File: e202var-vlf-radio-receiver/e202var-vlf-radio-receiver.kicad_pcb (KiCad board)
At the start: 2 copper layers, 55.9 x 81.3 mm, 49 parts, among them J1 9V, J2 ON/OFF, J3 HEADPHONES, J4 12V/18V, J5 FILTER, Q1 BC547, Q2 BC547, U1 MC7809, U2 TLE2426, U3 NJM386, U4 TL081CP

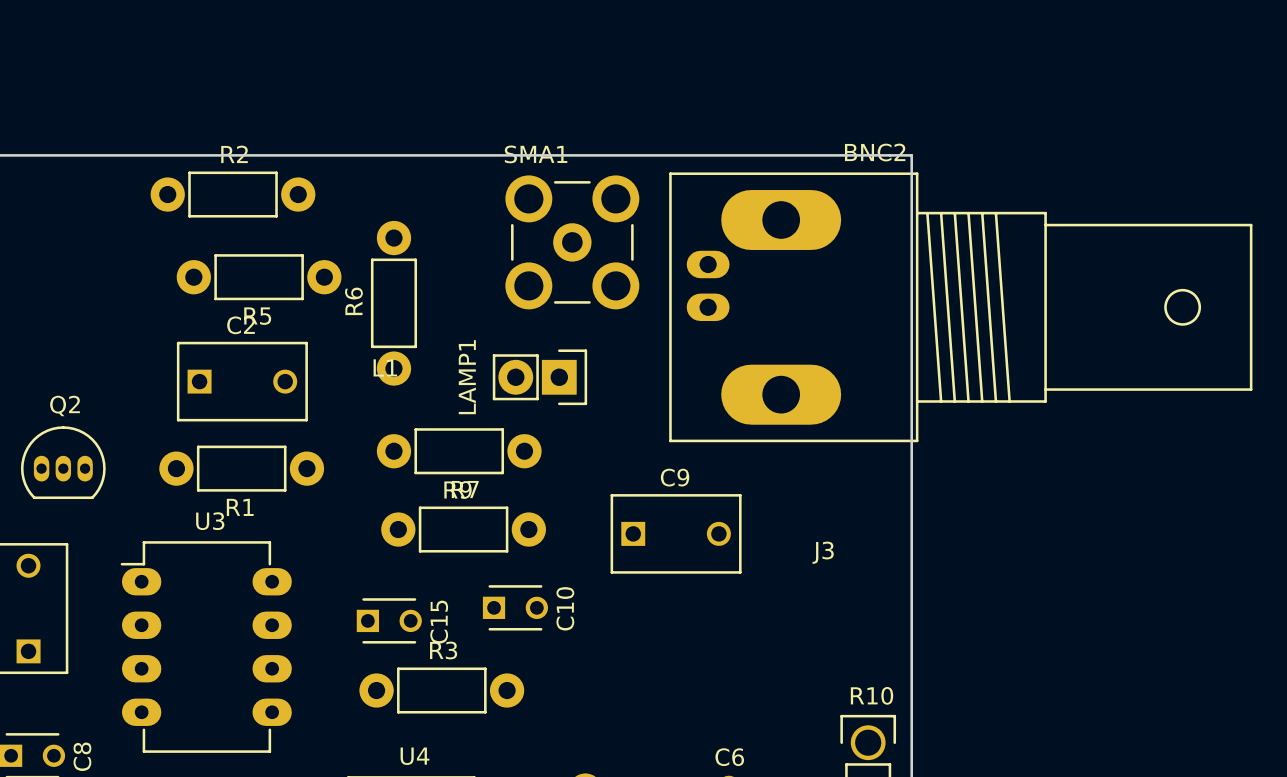
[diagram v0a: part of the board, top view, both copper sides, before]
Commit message: Added parts. Ready for layout.
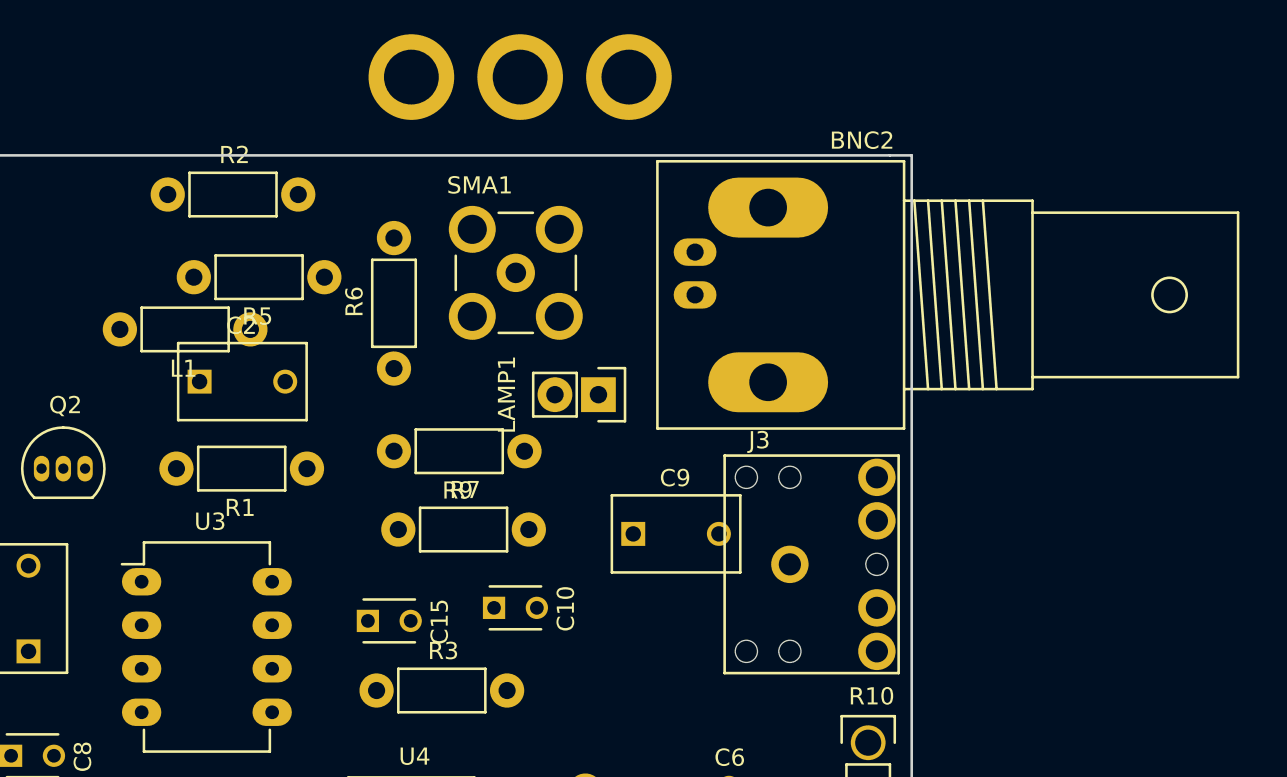
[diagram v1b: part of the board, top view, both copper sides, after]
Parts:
- added REF**: HOLE-PLATED-3.2MM, Wickerlib:HOLE-PLATED-3.2MM, F.Cu at (85.1, 33.5)
- added REF**: HOLE-PLATED-3.2MM, Wickerlib:HOLE-PLATED-3.2MM, F.Cu at (91.4, 33.5)
- added REF**: HOLE-PLATED-3.2MM, Wickerlib:HOLE-PLATED-3.2MM, F.Cu at (97.8, 33.5)
- L1: footprint Wickerlib:IND-78F-AXIAL -> Wickerlib:RES-CARBONFILM-7MM
- moved J3 4.32 mm to (107.2, 64.5)
- moved SMA1 3.75 mm to (91.2, 45.0)
- moved L1 2.65 mm to (75.7, 48.3), turned to 180 degrees
- moved LAMP1 2.50 mm to (96.0, 52.1)
- moved BNC2 1.05 mm to (106.7, 46.2)
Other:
- board text added: "12/9/2016"
- board text added: "E202VAR VLF Natural Radio Receiver"
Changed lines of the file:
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@@
 (kicad_pcb (version 4) (host pcbnew 4.0.4+e1-6308~48~ubuntu16.04.1-stable)
   (general
-    (links 87)
-    (no_connects 87)
-    (area 0 0 0 0)
+    (links 94)
+    (no_connects 94)
+    (area 58.343799 38.023799 114.376201 119.456201)
     (thickness 1.6)
-    (drawings 22)
+    (drawings 28)
     (tracks 0)
     (zones 0)
-    (modules 49)
+    (modules 52)
     (nets 33)
   )
@@
   )
   (module Wickerlib:CONN-BNC-TECONN-1-1634612-0 (layer F.Cu)
-    (at 107.4166 46.96968 270)
+    (at 106.6546 46.24578 270)
     (descr "BNC Socket TYCO AMP")
     (tags "BNC Socket TYCO AMP")
@@
       (net 29 "Net-(J1-Pad1)"))
   )
-  (module Wickerlib:SJ1-3523N (layer F.Cu)
-    (at 109.22 60.706)
-    (fp_text reference J3 (at 0 0.5) (layer F.SilkS)
-      (effects (font (size 1 1) (thickness 0.15)))
-    )
-    (fp_text value HEADPHONES (at 0 -0.5) (layer F.Fab)
-      (effects (font (size 1 1) (thickness 0.15)))
-    )
-  )
   (module Wickerlib:CONN-BARREL-JACK-2.5x5.5MM-TH (layer F.Cu)
     (at 90.651 109.5224 90)
@@
       (net 5 +2V))
   )
-  (module Wickerlib:IND-78F-AXIAL (layer F.Cu)
-    (at 76.454 50.8)
-    (fp_text reference L1 (at 7.112 -0.254) (layer F.SilkS)
-      (effects (font (size 1 1) (thickness 0.15)))
-    )
-    (fp_text value 3.3UH (at 0 -0.5) (layer F.Fab)
-      (effects (font (size 1 1) (thickness 0.15)))
-    )
-  )
   (module Wickerlib:CONN-HEADER-STRAIGHT-P2.54MM-1x02 (layer F.Cu)
-    (at 93.726 51.054 270)
+    (at 96.012 52.07 270)
     (descr "Through hole pin header")
     (tags "pin header")
@@
   )
   (module Wickerlib:CONN-SMA-STRAIGHT-TH (layer F.Cu)
-    (at 94.488 43.18)
+    (at 91.186 44.958)
     (descr "SMA pcb mounting jack")
     (tags "SMA Jack  Striaght")
@@
     (pad 8 thru_hole oval (at 7.62 0) (size 2.3 1.6) (drill 0.8) (layers *.Cu *.Mask F.SilkS))
   )
+  (module Wickerlib:RES-CARBONFILM-7MM (layer F.Cu)
+    (at 75.692 48.26 180)
+    (descr "Resistor, Axial,  RM 7.62mm, 1/3W,")
+    (tags "Resistor Axial RM 7.62mm 1/3W R3")
+    (fp_text reference L1 (at 3.8 0 180) (layer F.Fab)
+      (effects (font (size 1 1) (thickness 0.15)))
+    )
+    (fp_text value 3.3UH (at 3.81 3.81 180) (layer F.Fab) hide
+      (effects (font (size 1 1) (thickness 0.15)))
+    )
+    (fp_text user %R (at 3.9 -2.3 180) (layer F.SilkS)
+      (effects (font (size 1 1) (thickness 0.15)))
+    )
+    (fp_line (start 8.9 -1.5) (end -1.3 -1.5) (layer F.Fab) (width 0.0508))
+    (fp_line (start 8.9 1.5) (end 8.9 -1.5) (layer F.Fab) (width 0.0508))
+    (fp_line (start 8.8 1.5) (end 8.9 1.5) (layer F.Fab) (width 0.0508))
+    (fp_line (start -1.3 1.5) (end 8.8 1.5) (layer F.Fab) (width 0.0508))
+    (fp_line (start -1.3 -1.5) (end -1.3 1.5) (layer F.Fab) (width 0.0508))
+    (fp_line (start -1.25 -1.5) (end 8.85 -1.5) (layer F.CrtYd) (width 0.05))
+    (fp_line (start -1.25 1.5) (end -1.25 -1.5) (layer F.CrtYd) (width 0.05))
+    (fp_line (start 8.85 -1.5) (end 8.85 1.5) (layer F.CrtYd) (width 0.05))
+    (fp_line (start -1.25 1.5) (end 8.85 1.5) (layer F.CrtYd) (width 0.05))
+    (fp_line (start 1.27 -1.27) (end 6.35 -1.27) (layer F.SilkS) (width 0.15))
+    (fp_line (start 6.35 -1.27) (end 6.35 1.27) (layer F.SilkS) (width 0.15))
+    (fp_line (start 6.35 1.27) (end 1.27 1.27) (layer F.SilkS) (width 0.15))
+    (fp_line (start 1.27 1.27) (end 1.27 -1.27) (layer F.SilkS) (width 0.15))
+    (pad 1 thru_hole circle (at 0 0 180) (size 1.99898 1.99898) (drill 1.00076) (layers *.Cu *.SilkS *.Mask)
+      (net 3 "Net-(BNC2-Pad1)"))
+    (pad 2 thru_hole circle (at 7.62 0 180) (size 1.99898 1.99898) (drill 1.00076) (layers *.Cu *.SilkS *.Mask)
+      (net 7 "Net-(C2-Pad2)"))
+  )
+  (module Wickerlib:HOLE-PLATED-3.2MM (layer F.Cu)
+    (at 85.09 33.528)
+    (fp_text reference REF** (at 0 0) (layer F.Fab)
+      (effects (font (size 1 1) (thickness 0.15)))
+    )
+    (fp_text value HOLE-PLATED-3.2MM (at 0 -0.5) (layer F.Fab) hide
+      (effects (font (size 1 1) (thickness 0.15)))
+    )
+    (fp_circle (center 0 0) (end 2.54 1.27) (layer F.Fab) (width 0.04064))
+    (pad 1 thru_hole circle (at 0 0) (size 5 5) (drill 3.2) (layers *.Cu *.Mask))
+  )
+  (module Wickerlib:HOLE-PLATED-3.2MM (layer F.Cu)
+    (at 91.44 33.528)
+    (fp_text reference REF** (at 0 0) (layer F.Fab)
+      (effects (font (size 1 1) (thickness 0.15)))
+    )
+    (fp_text value HOLE-PLATED-3.2MM (at 0 -0.5) (layer F.Fab) hide
+      (effects (font (size 1 1) (thickness 0.15)))
+    )
+    (fp_circle (center 0 0) (end 2.54 1.27) (layer F.Fab) (width 0.04064))
+    (pad 1 thru_hole circle (at 0 0) (size 5 5) (drill 3.2) (layers *.Cu *.Mask))
+  )
+  (module Wickerlib:HOLE-PLATED-3.2MM (layer F.Cu)
+    (at 97.79 33.528)
+    (fp_text reference REF** (at 0 0) (layer F.Fab)
+      (effects (font (size 1 1) (thickness 0.15)))
+    )
+    (fp_text value HOLE-PLATED-3.2MM (at 0 -0.5) (layer F.Fab) hide
+      (effects (font (size 1 1) (thickness 0.15)))
+    )
+    (fp_circle (center 0 0) (end 2.54 1.27) (layer F.Fab) (width 0.04064))
+    (pad 1 thru_hole circle (at 0 0) (size 5 5) (drill 3.2) (layers *.Cu *.Mask))
+  )
+  (module Wickerlib:SJ1-3523N (layer F.Cu)
+    (at 107.188 64.516)
+    (fp_text reference J3 (at 1.27 -2.413) (layer F.Fab)
+      (effects (font (size 1 1) (thickness 0.15)))
+    )
+    (fp_text value HEADPHONES (at 0 -0.5) (layer F.Fab) hide
+      (effects (font (size 1 1) (thickness 0.15)))
+    )
+    (fp_text user %R (at -1.778 -9.779) (layer F.SilkS)
+      (effects (font (size 1 1) (thickness 0.15)))
+    )
+    (fp_line (start -3.81 3.81) (end 6.35 3.81) (layer F.CrtYd) (width 0.04064))
+    (fp_line (start -3.81 -8.89) (end -3.81 3.81) (layer F.CrtYd) (width 0.04064))
+    (fp_line (start 6.35 -8.89) (end -3.81 -8.89) (layer F.CrtYd) (width 0.04064))
+    (fp_line (start 6.35 3.81) (end 6.35 -8.89) (layer F.CrtYd) (width 0.04064))
+    (fp_line (start -3.81 3.81) (end 6.35 3.81) (layer F.Fab) (width 0.04064))
+    (fp_line (start -3.81 -8.89) (end -3.81 3.81) (layer F.Fab) (width 0.04064))
+    (fp_line (start 6.35 -8.89) (end -3.81 -8.89) (layer F.Fab) (width 0.04064))
+    (fp_line (start 6.35 -8.89) (end 6.35 3.81) (layer F.Fab) (width 0.04064))
+    (fp_line (start -3.81 3.81) (end 6.35 3.81) (layer F.SilkS) (width 0.1524))
+    (fp_line (start -3.81 -8.89) (end -3.81 3.81) (layer F.SilkS) (width 0.1524))
+    (fp_line (start 6.35 -8.89) (end -3.81 -8.89) (layer F.SilkS) (width 0.1524))
+    (fp_line (start 6.35 3.81) (end 6.35 -8.89) (layer F.SilkS) (width 0.1524))
+    (pad 4 thru_hole circle (at 5.08 -7.62) (size 2.1844 2.1844) (drill 1.2954) (layers *.Cu *.Mask)
+      (net 1 GND))
+    (pad 3 thru_hole circle (at 5.08 -5.08) (size 2.1844 2.1844) (drill 1.2954) (layers *.Cu *.Mask)
+      (net 1 GND))
+    (pad "" np_thru_hole circle (at 5.08 -2.54) (size 1.2954 1.2954) (drill 1.2954) (layers *.Cu))
+    (pad 2 thru_hole circle (at 5.08 0) (size 2.1844 2.1844) (drill 1.2954) (layers *.Cu *.Mask)
+      (net 17 "Net-(C9-Pad1)"))
+    (pad 1 thru_hole circle (at 5.08 2.54) (size 2.1844 2.1844) (drill 1.2954) (layers *.Cu *.Mask)
+      (net 17 "Net-(C9-Pad1)"))
+    (pad 5 thru_hole circle (at 0 -2.54) (size 2.1844 2.1844) (drill 1.2954) (layers *.Cu *.Mask)
+      (net 1 GND))
+    (pad "" np_thru_hole circle (at 0 -7.62) (size 1.2954 1.2954) (drill 1.2954) (layers *.Cu))
+    (pad "" np_thru_hole circle (at -2.54 -7.62) (size 1.2954 1.2954) (drill 1.2954) (layers *.Cu))
+    (pad "" np_thru_hole circle (at 0 2.54) (size 1.2954 1.2954) (drill 1.2954) (layers *.Cu))
+    (pad "" np_thru_hole circle (at -2.54 2.54) (size 1.2954 1.2954) (drill 1.2954) (layers *.Cu))
+  )
+  (gr_text 12/9/2016 (at 109.22 30.734) (layer F.Fab)
+    (effects (font (size 1.016 1.016) (thickness 0.1524)))
+  )
+  (gr_text "E202VAR VLF Natural Radio Receiver" (at 99.568 28.702) (layer F.Fab)
+    (effects (font (size 1.016 1.016) (thickness 0.1524)))
+  )
+  (gr_line (start 58.42 38.1) (end 114.3 38.1) (layer F.Fab) (width 0.1524))
+  (gr_line (start 58.42 119.38) (end 58.42 38.1) (layer F.Fab) (width 0.1524))
+  (gr_line (start 114.3 119.38) (end 58.42 119.38) (layer F.Fab) (width 0.1524))
+  (gr_line (start 114.3 38.1) (end 114.3 119.38) (layer F.Fab) (width 0.1524))
   (gr_line (start 113.03 38.1) (end 114.3 38.1) (layer Edge.Cuts) (width 0.1524))
   (gr_line (start 58.42 38.1) (end 113.03 38.1) (layer Edge.Cuts) (width 0.1524))
